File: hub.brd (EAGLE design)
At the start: 160 x 100 mm, 27 parts, among them U1 10118194-MICRO-USB, U2 LM3671MF-3.3/NOPBMF05A-M, U3 SN74LVC1T45DBVRDBV6-M, U4 SN74LVC1T45DBVRDBV6-M

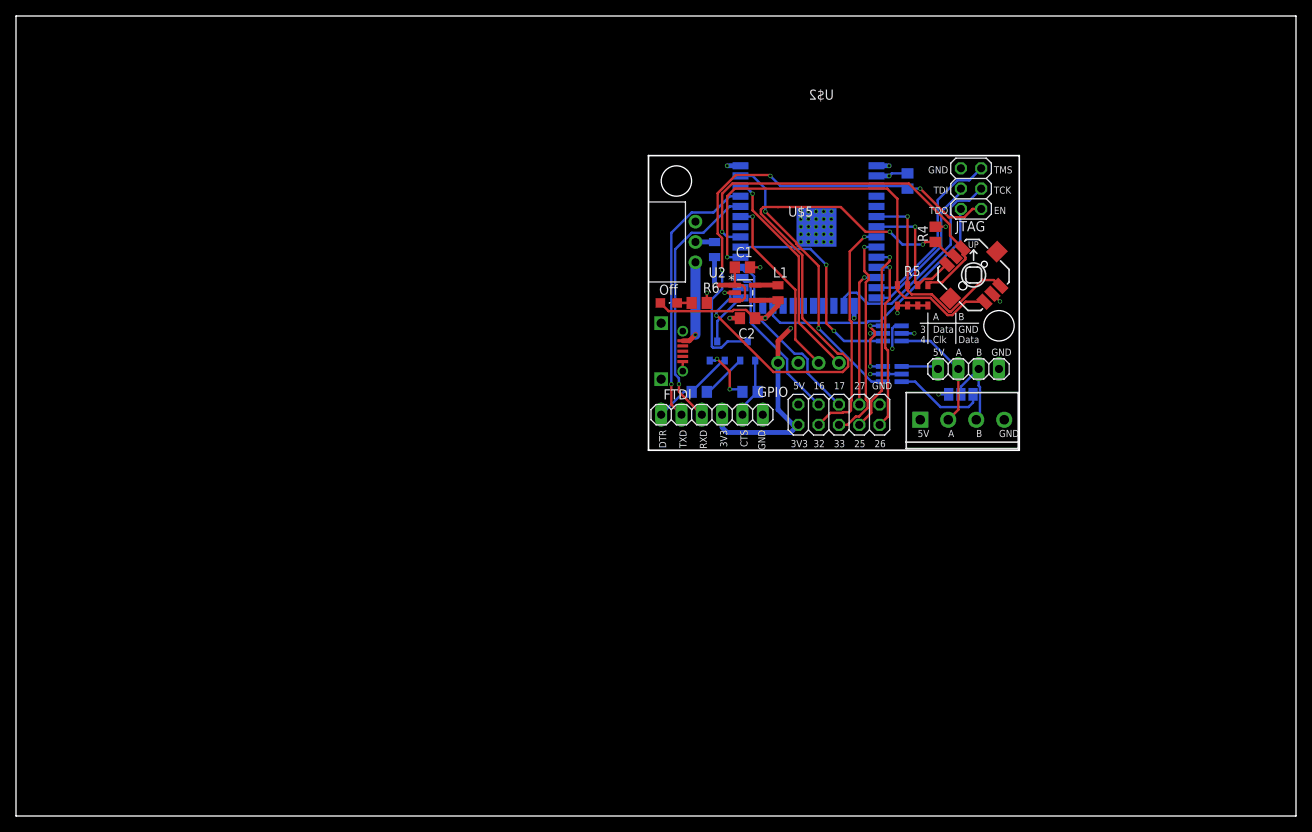
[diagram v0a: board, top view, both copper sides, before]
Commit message: Final tweaks and BOM creation
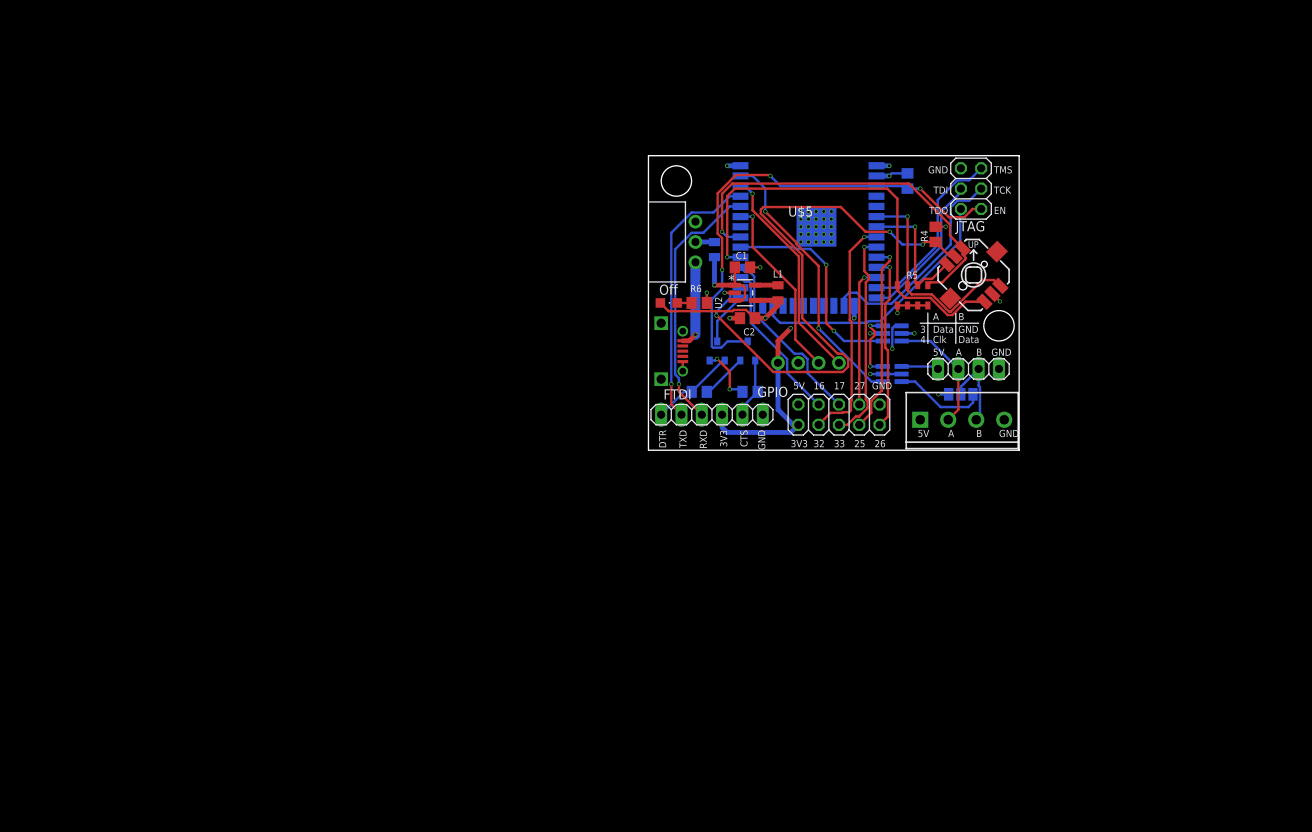
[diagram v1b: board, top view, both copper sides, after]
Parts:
- renumbered U$1 to U5, U$4 to U6
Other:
- board size 160 x 100 mm -> 46.3 x 36.8 mm
- board text added: "RVL Controller v1.0 Copyright Bryan Hughes October 2019"
